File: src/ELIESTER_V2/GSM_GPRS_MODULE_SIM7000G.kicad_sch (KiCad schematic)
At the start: 53 parts, among them J5 SIM_Card, Q11 MMBT3904, Q12 MMBT3904, Q5 BSN20, SW3 SW_Push, U2 SIM7000G

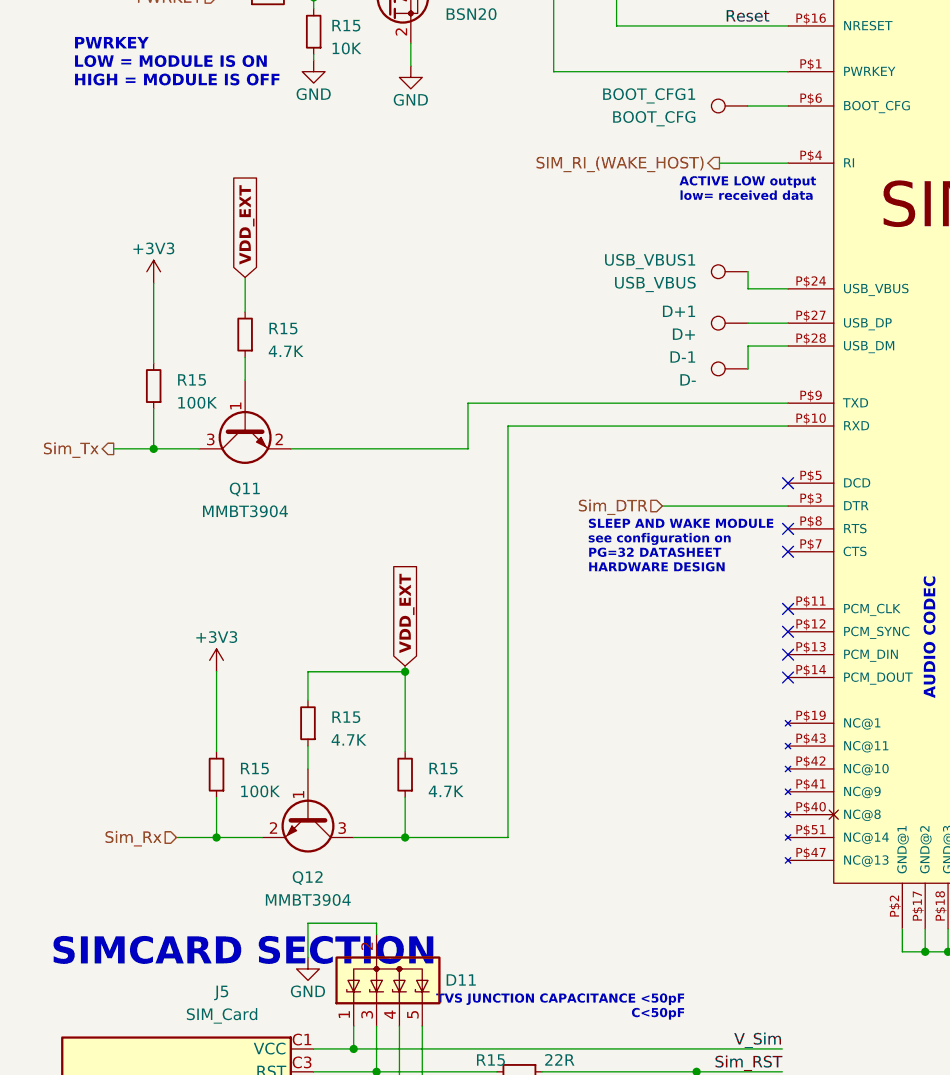
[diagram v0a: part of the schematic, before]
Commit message: schematic update and gerber updates with corrections
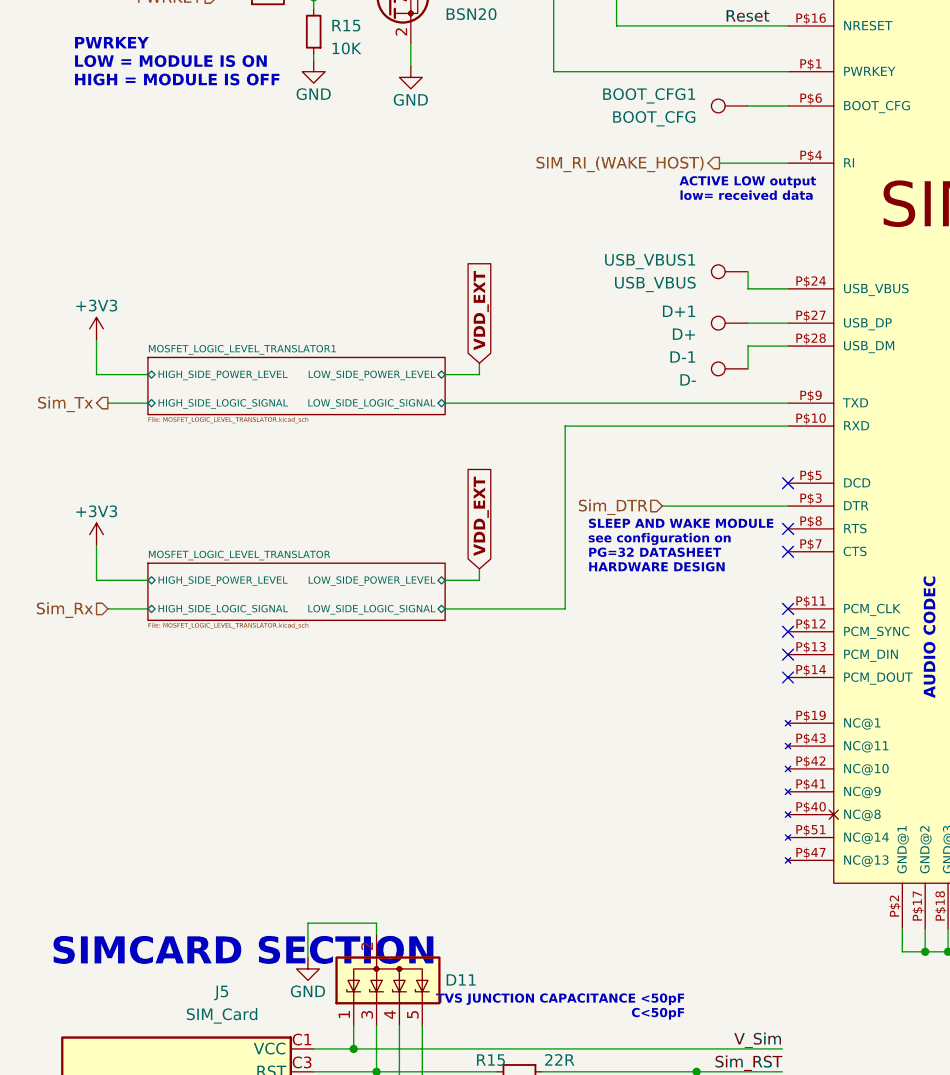
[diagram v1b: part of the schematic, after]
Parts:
- removed Q11, Q12: MMBT3904, Package_TO_SOT_SMD:SOT-23, symbol Transistor_BJT:MMBT3904
- removed R15 (x2): 100K, Resistor_SMD:R_0603_1608Metric, symbol Device:R_Small
- removed R15 (x3): 4.7K, Resistor_SMD:R_0603_1608Metric, symbol Device:R_Small
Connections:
- net MOSFET_LOGIC_LEVEL_TRANSLATOR/LOW_SIDE_LOGIC_SIGNAL: now reaches U2.P$10 (RXD)
- net MOSFET_LOGIC_LEVEL_TRANSLATOR1/LOW_SIDE_LOGIC_SIGNAL: now reaches U2.P$9 (TXD)
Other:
- added sheet MOSFET_LOGIC_LEVEL_TRANSLATOR (MOSFET_LOGIC_LEVEL_TRANSLATOR.kicad_sch)
- added sheet MOSFET_LOGIC_LEVEL_TRANSLATOR1 (MOSFET_LOGIC_LEVEL_TRANSLATOR.kicad_sch)
